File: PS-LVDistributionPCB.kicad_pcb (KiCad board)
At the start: 2 copper layers, 166.5 x 58.5 mm, 41 parts, among them J1 Conn_01x02, J10 Conn_01x02, J11 Conn_01x02, J12 Conn_01x02, J13 Conn_01x02, J14 Conn_01x02, J15 Conn_01x20, J2 Conn_01x02, J3 Conn_01x02, J4 Conn_01x02, J5 Conn_01x02, J6 Conn_01x02, J7 Conn_01x02, J8 Conn_01x02, J9 Conn_01x02

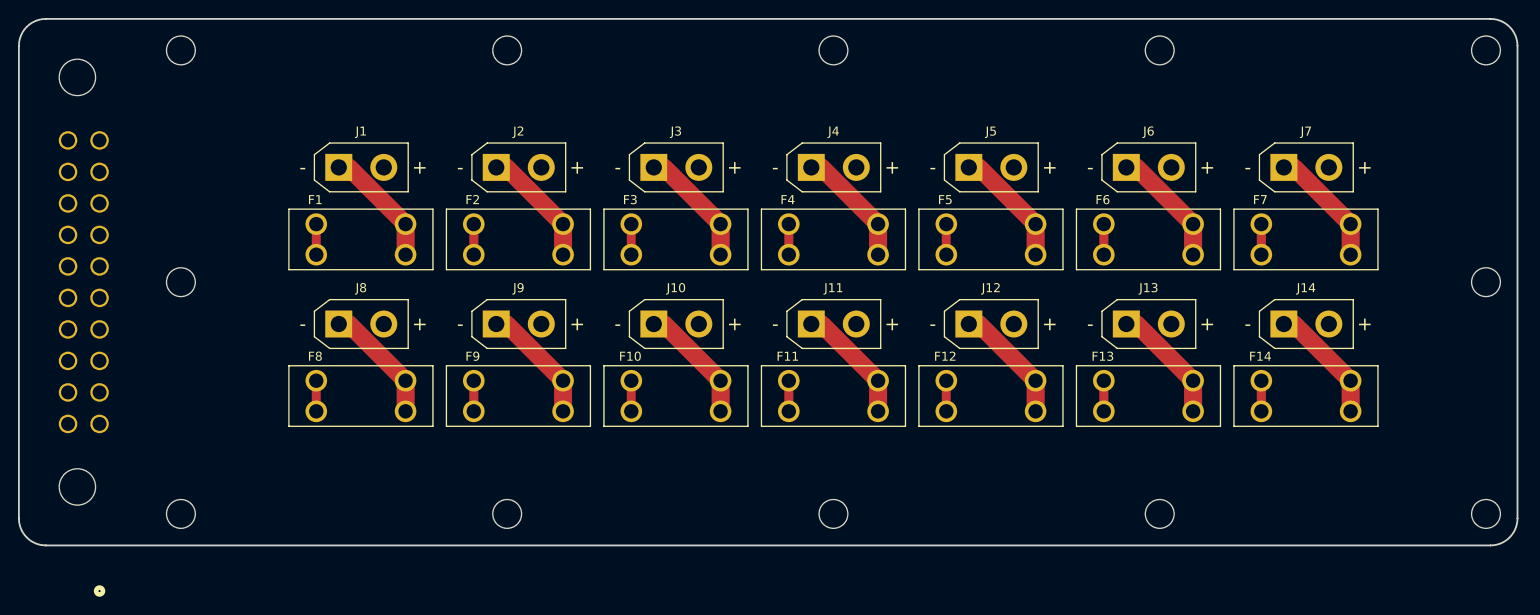
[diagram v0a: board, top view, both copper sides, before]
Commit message: common gnd
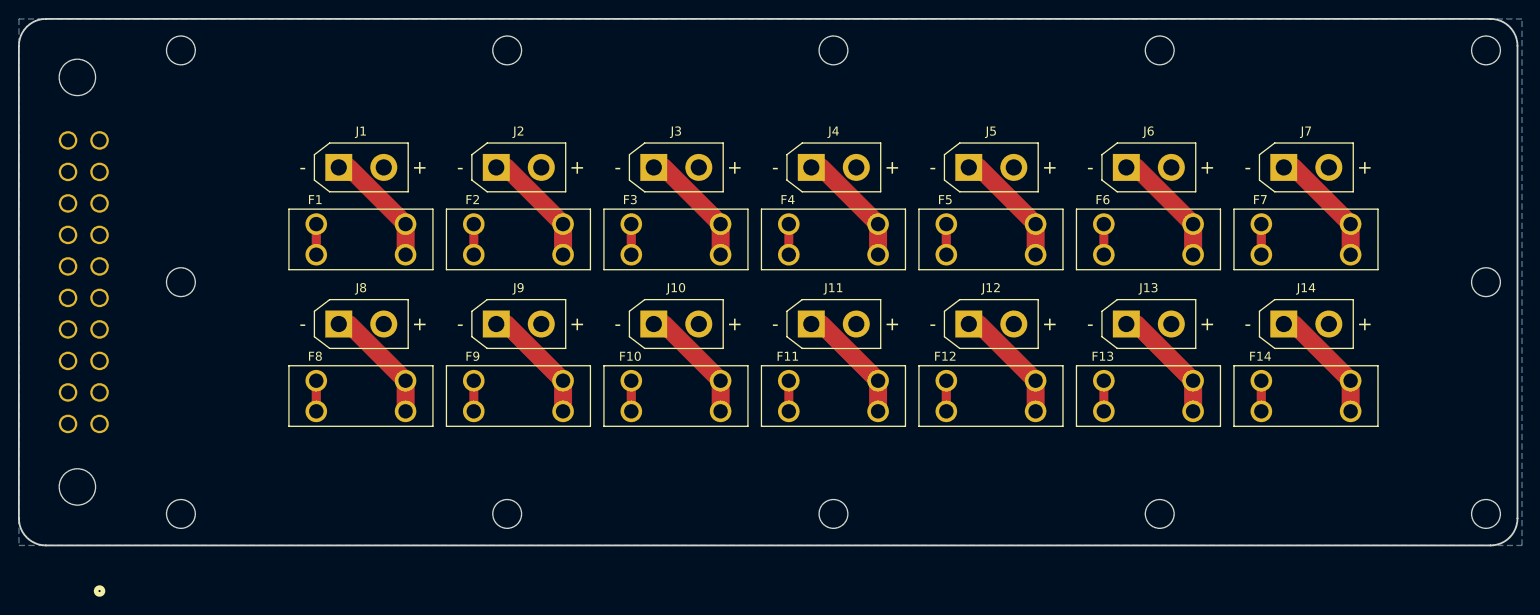
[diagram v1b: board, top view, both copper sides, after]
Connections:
- J1 pad 2: GND1 -> GND
- J10 pad 2: GND4 -> GND
- J11 pad 2: GND5 -> GND
- J12 pad 2: GND5 -> GND
- J13 pad 2: GND6 -> GND
- J14 pad 2: GND6 -> GND
- J15 pad 15: GND1 -> GND
- J15 pad 16: GND2 -> GND
- J15 pad 17: GND3 -> GND
- J15 pad 18: GND4 -> GND
- J15 pad 19: GND5 -> GND
- J15 pad 20: GND6 -> GND
- J2 pad 2: GND1 -> GND
- J3 pad 2: GND1 -> GND
- J4 pad 2: GND2 -> GND
- J5 pad 2: GND2 -> GND
- J6 pad 2: GND3 -> GND
- J7 pad 2: GND3 -> GND
- J8 pad 2: GND3 -> GND
- J9 pad 2: GND4 -> GND
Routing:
- added copper zone on B.Cu, net GND
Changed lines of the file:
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@@
 	(net 26 "P13")
 	(net 27 "P14")
-	(net 28 "GND6")
-	(net 29 "GND3")
-	(net 30 "GND2")
-	(net 31 "GND1")
-	(net 32 "GND5")
-	(net 33 "GND4")
-	(net 34 "Net-(J1-Pin_1)")
+	(net 28 "GND")
+	(net 29 "Net-(J1-Pin_1)")
 	(footprint "MountingHole:MountingHole_3.2mm_M3"
 		(layer "F.Cu")
@@
 			(layers "*.Cu" "*.Mask")
 			(remove_unused_layers no)
-			(net 30 "GND2")
+			(net 28 "GND")
 			(pinfunction "Pin_2")
 			(pintype "passive")
@@
 			(layers "*.Cu" "*.Mask")
 			(remove_unused_layers no)
-			(net 32 "GND5")
+			(net 28 "GND")
 			(pinfunction "Pin_2")
 			(pintype "passive")
@@
 			(layers "*.Cu" "*.Mask")
 			(remove_unused_layers no)
-			(net 34 "Net-(J1-Pin_1)")
+			(net 29 "Net-(J1-Pin_1)")
 			(pinfunction "Pin_1")
 			(pintype "passive")
@@
 			(layers "*.Cu" "*.Mask")
 			(remove_unused_layers no)
-			(net 31 "GND1")
+			(net 28 "GND")
 			(pinfunction "Pin_2")
 			(pintype "passive")
@@
 			(layers "*.Cu" "*.Mask")
 			(remove_unused_layers no)
-			(net 33 "GND4")
+			(net 28 "GND")
 			(pinfunction "Pin_2")
 			(pintype "passive")
@@
 			(layers "*.Cu" "*.Mask")
 			(remove_unused_layers no)
-			(net 29 "GND3")
+			(net 28 "GND")
 			(pinfunction "Pin_2")
 			(pintype "passive")
@@
 			(layers "*.Cu" "*.Mask")
 			(remove_unused_layers no)
-			(net 30 "GND2")
+			(net 28 "GND")
 			(pinfunction "Pin_2")
 			(pintype "passive")
@@
 			(layers "*.Cu" "*.Mask")
 			(remove_unused_layers no)
-			(net 28 "GND6")
+			(net 28 "GND")
 			(pinfunction "Pin_2")
 			(pintype "passive")
@@
 			(layers "*.Cu" "*.Mask")
 			(remove_unused_layers no)
-			(net 28 "GND6")
+			(net 28 "GND")
 			(pinfunction "Pin_2")
 			(pintype "passive")
@@
 			(layers "*.Cu" "*.Mask")
 			(remove_unused_layers no)
-			(net 33 "GND4")
+			(net 28 "GND")
 			(pinfunction "Pin_2")
 			(pintype "passive")
@@
 			(layers "*.Cu" "*.Mask")
 			(remove_unused_layers no)
-			(net 31 "GND1")
+			(net 28 "GND")
 			(pinfunction "Pin_2")
 			(pintype "passive")
@@
 			(layers "*.Cu" "*.Mask")
 			(remove_unused_layers no)
-			(net 34 "Net-(J1-Pin_1)")
+			(net 29 "Net-(J1-Pin_1)")
 			(pintype "passive")
 			(solder_mask_margin 0.102)
@@
 			(layers "*.Cu" "*.Mask")
 			(remove_unused_layers no)
-			(net 34 "Net-(J1-Pin_1)")
+			(net 29 "Net-(J1-Pin_1)")
 			(pintype "passive")
 			(solder_mask_margin 0.102)
@@
 			(layers "*.Cu" "*.Mask")
 			(remove_unused_layers no)
-			(net 32 "GND5")
+			(net 28 "GND")
 			(pinfunction "Pin_2")
 			(pintype "passive")
@@
 			(layers "*.Cu" "*.Mask")
 			(remove_unused_layers no)
-			(net 29 "GND3")
+			(net 28 "GND")
 			(pinfunction "Pin_2")
 			(pintype "passive")
@@
 			(layers "*.Cu" "*.Mask")
 			(remove_unused_layers no)
-			(net 29 "GND3")
+			(net 28 "GND")
 			(pinfunction "Pin_2")
 			(pintype "passive")
@@
 			(layers "*.Cu" "*.Mask")
 			(remove_unused_layers no)
-			(net 31 "GND1")
+			(net 28 "GND")
 			(pinfunction "Pin_2")
 			(pintype "passive")
@@
 			(layers "*.Cu" "*.Mask")
 			(remove_unused_layers no)
-			(net 31 "GND1")
+			(net 28 "GND")
 			(pinfunction "Pin_15")
 			(pintype "passive")
@@
 			(layers "*.Cu" "*.Mask")
 			(remove_unused_layers no)
-			(net 30 "GND2")
+			(net 28 "GND")
 			(pinfunction "Pin_16")
 			(pintype "passive")
@@
 			(layers "*.Cu" "*.Mask")
 			(remove_unused_layers no)
-			(net 29 "GND3")
+			(net 28 "GND")
 			(pinfunction "Pin_17")
 			(pintype "passive")
@@
 			(layers "*.Cu" "*.Mask")
 			(remove_unused_layers no)
-			(net 33 "GND4")
+			(net 28 "GND")
 			(pinfunction "Pin_18")
 			(pintype "passive")
@@
 			(layers "*.Cu" "*.Mask")
 			(remove_unused_layers no)
-			(net 32 "GND5")
+			(net 28 "GND")
 			(pinfunction "Pin_19")
 			(pintype "passive")
@@
 			(layers "*.Cu" "*.Mask")
 			(remove_unused_layers no)
-			(net 28 "GND6")
+			(net 28 "GND")
 			(pinfunction "Pin_20")
 			(pintype "passive")
@@
 		(width 1)
 		(layer "F.Cu")
-		(net 34)
+		(net 29)
 	)
 	(segment
@@
 		(width 2)
 		(layer "F.Cu")
-		(net 34)
+		(net 29)
 	)
 	(segment
@@
 		(width 2)
 		(layer "F.Cu")
-		(net 34)
+		(net 29)
+	)
+	(zone
+		(net 28)
+		(net_name "GND")
+		(layer "B.Cu")
+		(hatch edge 0.5)
+		(connect_pads yes
+			(clearance 0.5)
+		)
+		(min_thickness 0.25)
+		(filled_areas_thickness no)
+		(fill yes
+			(thermal_gap 0.5)
+			(thermal_bridge_width 0.5)
+		)
+		(polygon
+			(pts
+				(xy 86 58) (xy 86 116.5) (xy 253 116.5) (xy 253 58)
+			)
+		)
 	)
 	(group "Replicated Group ['/Power Output5/']"
